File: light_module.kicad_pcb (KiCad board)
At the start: 2 copper layers, 50 x 50 mm, 23 parts, among them J1 Conn_01x03_Pin, J2 Conn_01x03_Pin, U1 AL8860MP

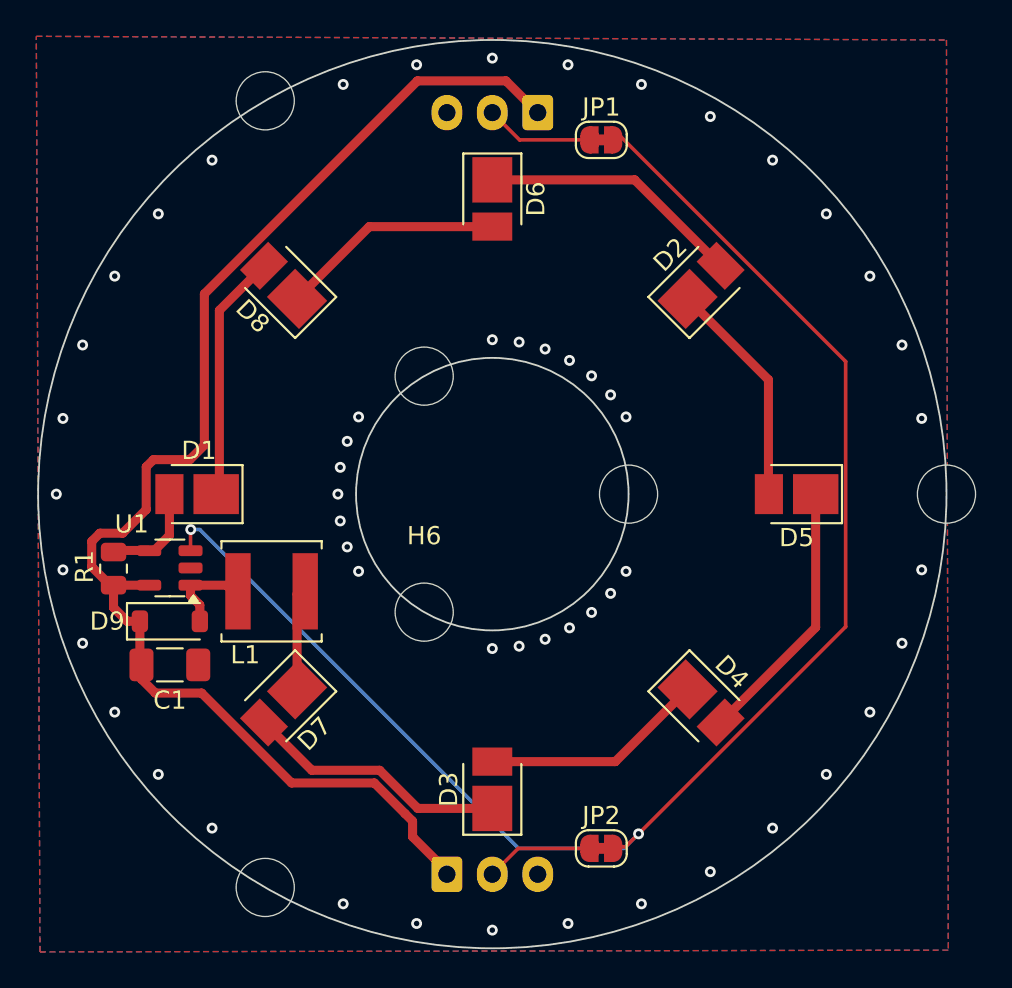
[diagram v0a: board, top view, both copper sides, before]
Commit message: round
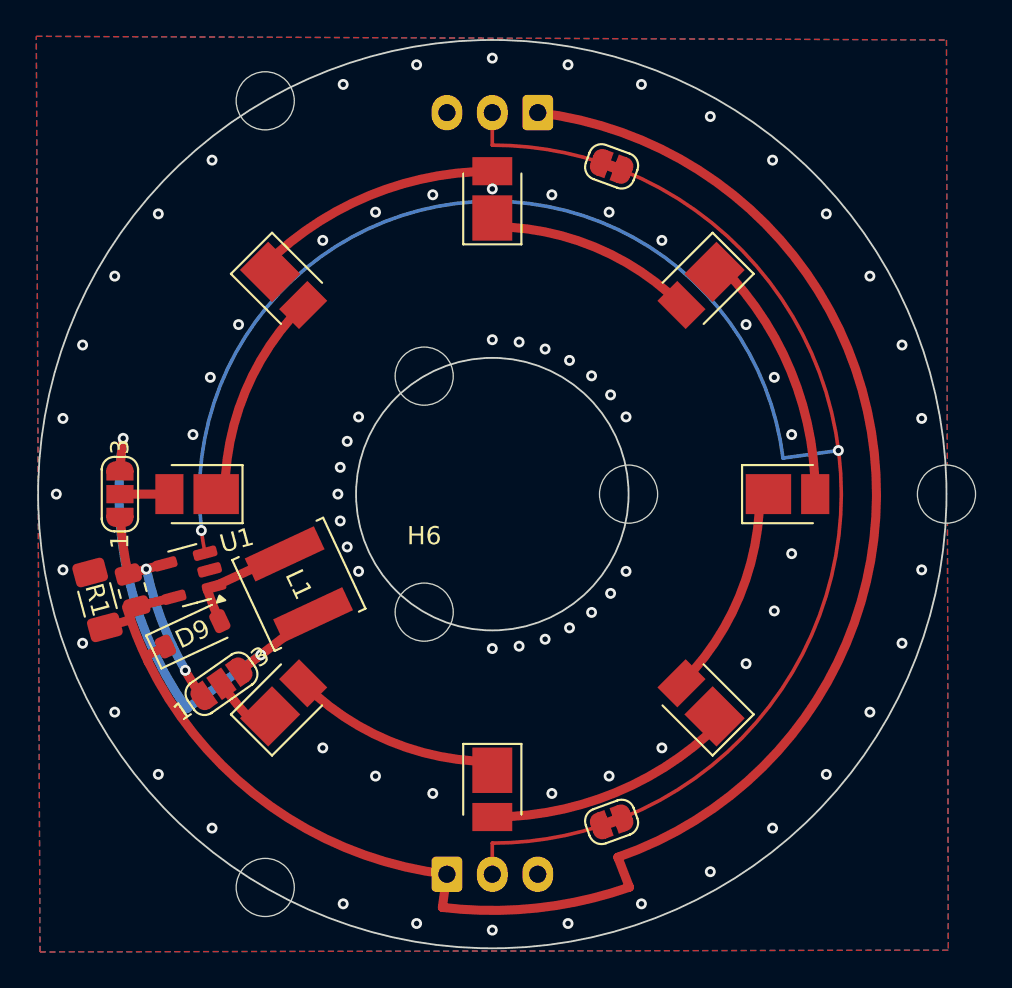
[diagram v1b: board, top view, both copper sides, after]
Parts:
- added JP3: SolderJumper_3_Open, Jumper:SolderJumper-3_P1.3mm_Open_RoundedPad1.0x1.5mm_NumberLabels, F.Cu at (121.5, 100.0)
- added JP4: SolderJumper_3_Open, Jumper:SolderJumper-3_P1.3mm_Open_RoundedPad1.0x1.5mm_NumberLabels, F.Cu at (127.1, 110.4)
- moved D2 32.5 mm to (130.5, 111.5)
- moved D7 30.0 mm to (142.0, 83.8), turned to 90 degrees
- moved D6 12.4 mm to (153.5, 88.5), turned to -135 degrees
- moved C1 5.35 mm to (120.3, 105.8), turned to 105 degrees
- moved R1 1.60 mm to (122.2, 105.3), turned to -75 degrees
- moved JP1 1.56 mm to (148.6, 82.0), turned to -20 degrees
- moved JP2 1.56 mm to (148.6, 118.0), turned to 20 degrees
- moved L1 1.55 mm to (131.4, 105.0), turned to 115 degrees
- moved D9 1.43 mm to (125.5, 107.7), turned to 25 degrees
- moved U1 1.16 mm to (125.3, 104.5), turned to -165 degrees
- moved D5 0.50 mm to (158.2, 100.0), turned to 0 degrees
- turned D3 to -90 degrees
- turned D4 to 135 degrees
- turned D8 to -45 degrees
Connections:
- D1 pad 2: /V_LED -> /LED_ANODE
- D2 pad 1: Net-(D2-K) -> /LED_KATHODE
- D3 pad 1: Net-(D3-K) -> Net-(D2-A)
- D5 pad 2: Net-(D2-K) -> Net-(D5-A)
- D6 pad 1: Net-(D2-A) -> Net-(D5-A)
- D7 pad 1: /KATHODE_LED -> Net-(D6-A)
- D7 pad 2: Net-(D3-K) -> Net-(D7-A)
- D8 pad 1: Net-(D6-A) -> Net-(D7-A)
- L1 pad 1: /KATHODE_LED -> /V-_LED
- R1 pad 1: /V_LED -> /V+_LED
- U1 pad 4: /V_LED -> /V+_LED
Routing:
- net /CTRL: track 83.7 -> 3.08 mm
- net +24V: track 75.3 -> 8.78 mm
- net Net-(D4-A): track 14.7 -> 0.04 mm
- net Net-(D3-K): track 14.5 -> 0.00 mm
- net Net-(D2-A): track 14.5 -> 0.00 mm
- net Net-(D1-K): track 14.0 -> 0.62 mm
- net Net-(D2-K): track 12.6 -> 0.00 mm
- net Net-(D6-A): track 12.4 -> 0.00 mm
- net Net-(D3-A): track 12.4 -> 0.00 mm
- net /V-_LED: track 0.00 -> 10.1 mm, vias 0 -> 2
- net /V_LED: track 5.74 -> 0.00 mm
- net /KATHODE_LED: track 5.53 -> 0.00 mm
- net Net-(J1-Pin_2): track 5.91 -> 1.71 mm
- net Net-(J2-Pin_2): track 5.97 -> 1.79 mm
- net /LED_ANODE: track 0.00 -> 2.72 mm
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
